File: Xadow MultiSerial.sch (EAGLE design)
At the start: 45 parts, among them J1 12p 0.5mm bottom contact, J2 12p 0.5mm bottom contact, J3 12p 0.5mm bottom contact, J4 12p 0.5mm bottom contact, Q1 MOSFET-N-044020001, Q2 MOSFET-N-044020001, Q3 MOSFET-N-044020001, Q4 MOSFET-N-044020001, Q5 MOSFET-N-044020001, Q6 MOSFET-N-044020001, U1 SC16IS752, X1 CTS_32X25_SMD

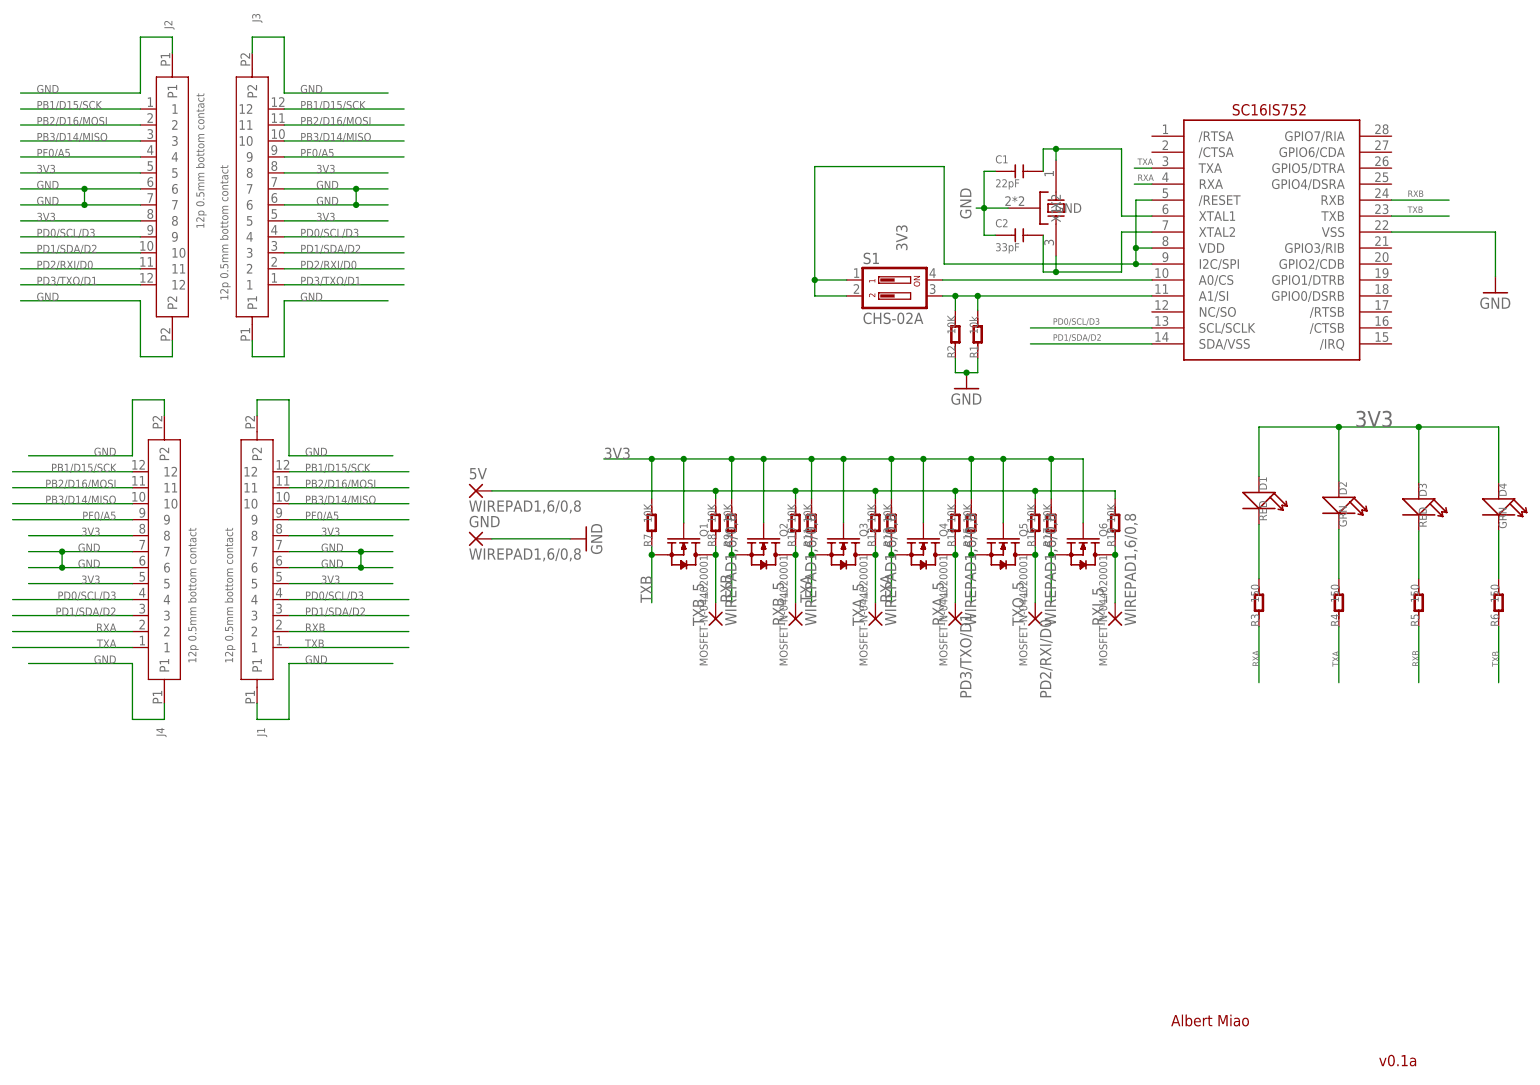
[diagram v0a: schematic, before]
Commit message: Fixed errors and relayed out, last attempt with MOSFET level shifter, need to try TXS shifter
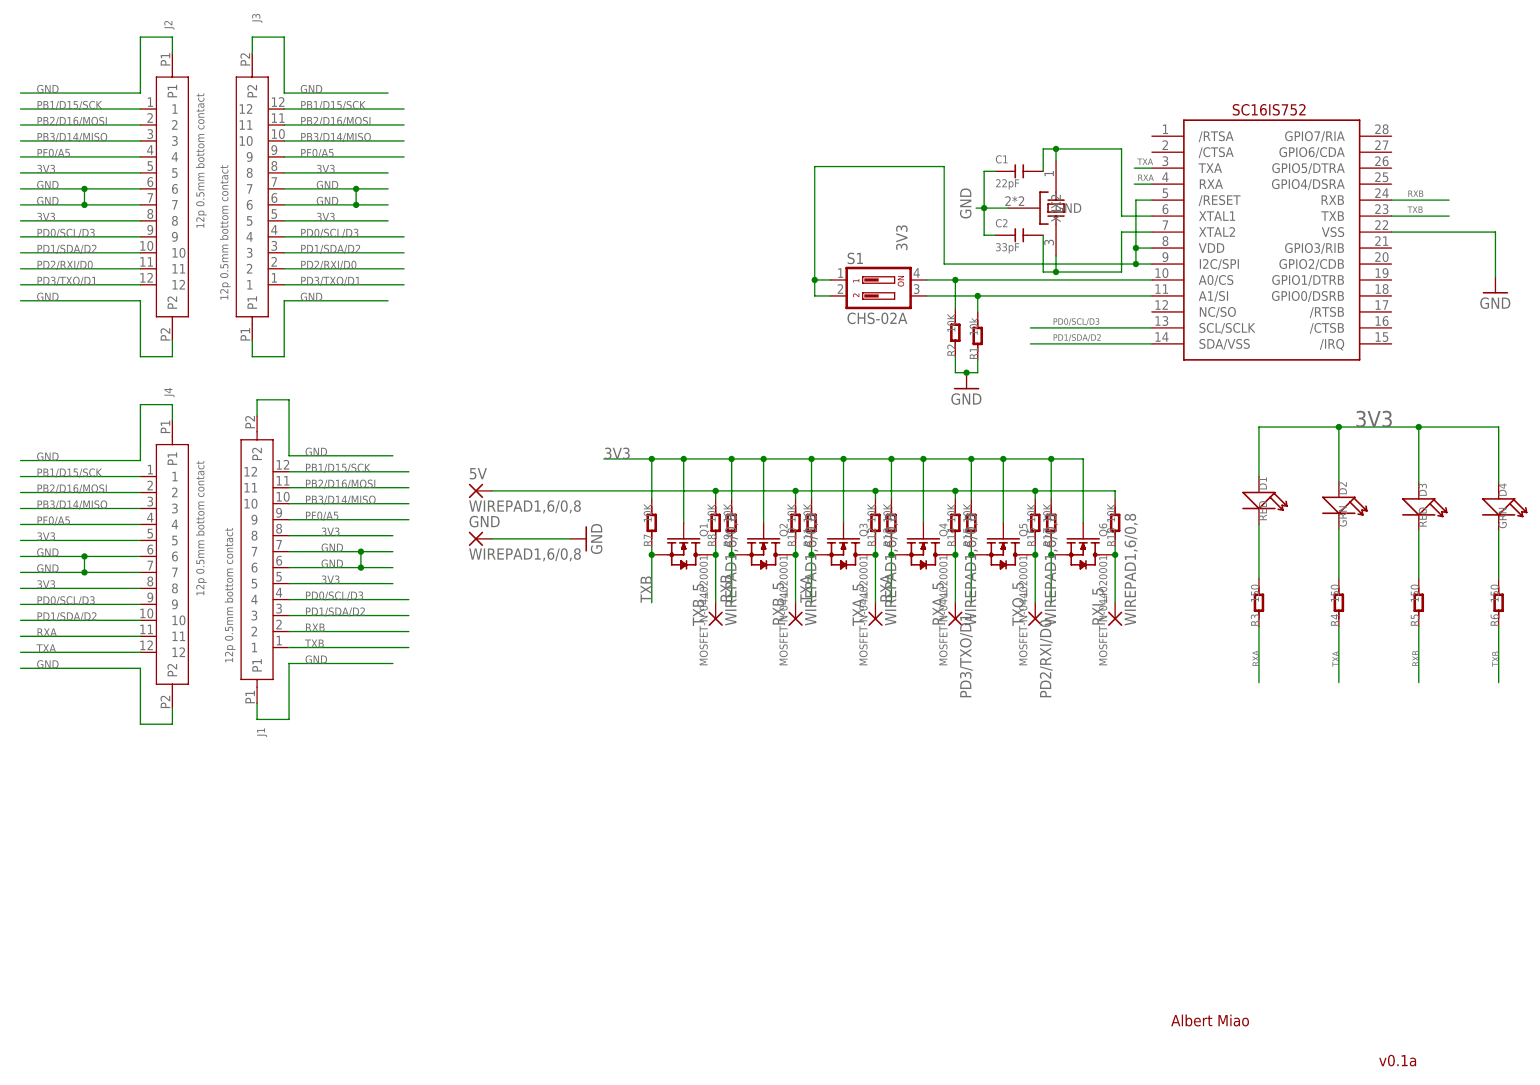
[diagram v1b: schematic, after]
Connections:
- net N$3: no longer R2.2
- net N$5: now also R2.2
- net PB1/D15/SCK: now also J4.1; no longer J4.12
- net PB2/D16/MOSI: now also J4.2; no longer J4.11
- net PB3/D14/MISO: now also J4.3; no longer J4.10
- net PD0/SCL/D3: now also J4.9; no longer J4.4
- net PD1/SDA/D2: now also J4.10; no longer J4.3
- net PF0/A5: now also J4.4; no longer J4.9
- net RXA: now also J4.11; no longer J4.2
- net TXA: now also J4.12; no longer J4.1
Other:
- moved on the sheet: J4, S1

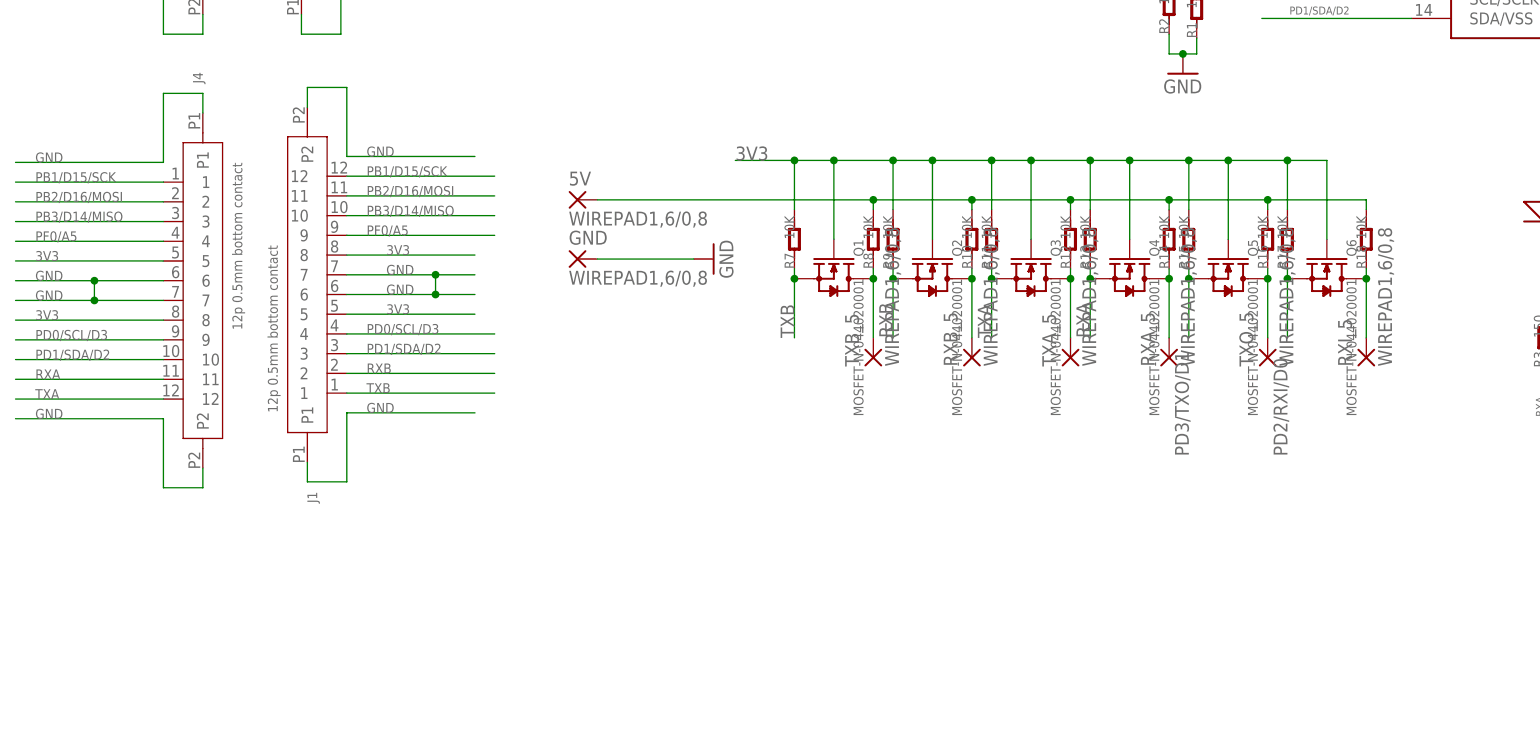
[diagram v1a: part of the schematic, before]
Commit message: Added TXS based level translation
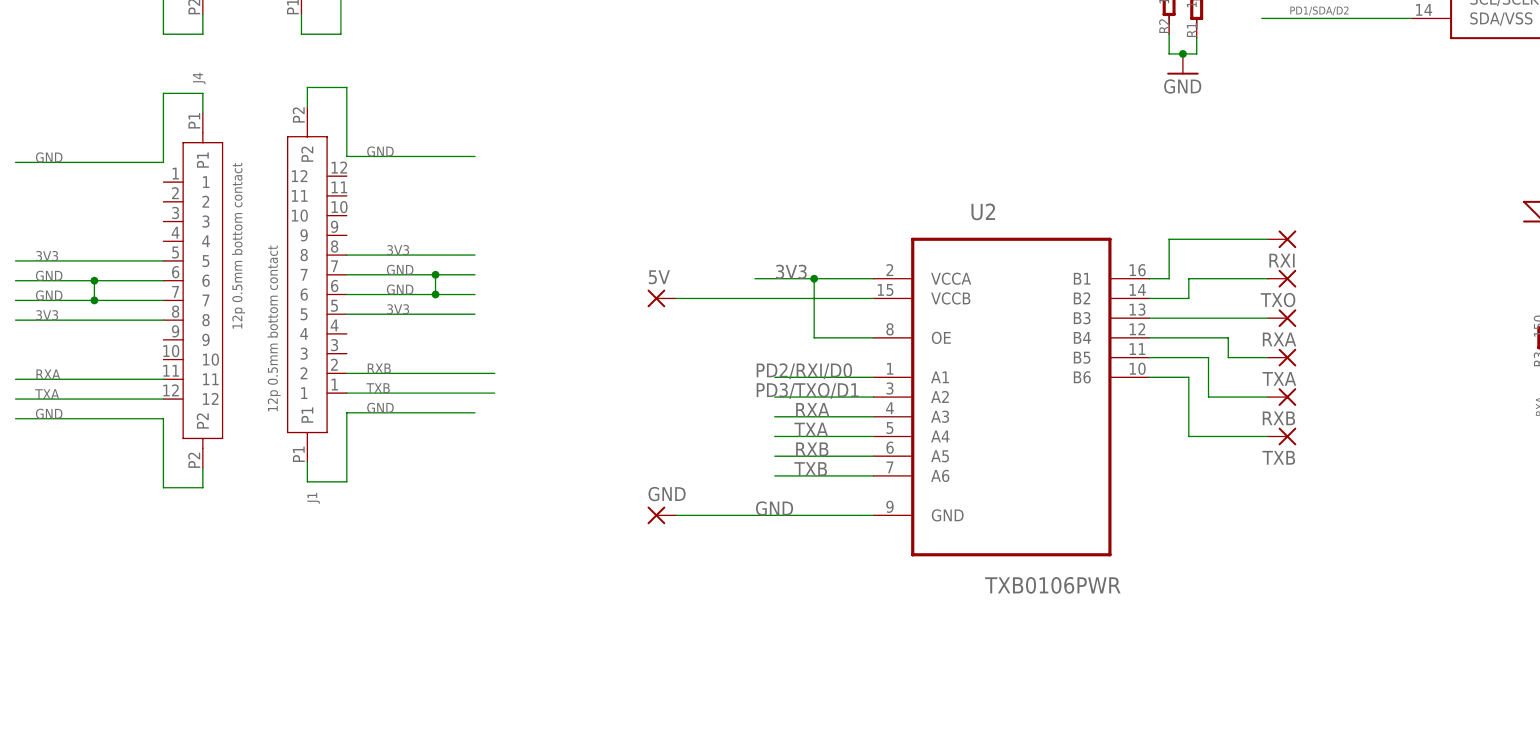
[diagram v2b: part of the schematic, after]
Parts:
- removed Q1, Q2, Q3, Q4, Q5, Q6: MOSFET-N-044020001, OPL:MOSFET-N-044020001
- removed R10, R11, R12, R13, R14, R15, R16, R17, R18, R7, R8, R9: 10K, OPL:R-0603
- removed RXA_5, RXB_5, RXI_5, TXA_5, TXB_5, TXO_5: WIREPAD1,6/0,8, wirepad:WIREPAD1,6/0,8
- added RXA, RXB, RXI, TXA, TXB, TXO: (no value), wirepad:1,6/0,8
- added U2: TXB0106PWR, Texas Instruments_By_element14_Batch_1:TXB0106PWR
- 5V, GND: value WIREPAD1,6/0,8 -> (none); device wirepad:WIREPAD1,6/0,8 -> wirepad:1,6/0,8
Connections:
- removed net N$17: 5V.P, R10.2, R12.2, R14.2, R16.2, R18.2, R8.2
- new net N$4: 5V.P, U2.VCCB
- net 3V3: now also U2.OE, U2.VCCA; no longer Q1.G, Q2.G, Q3.G, Q4.G, Q5.G, Q6.G, R11.2, R13.2, R15.2, R17.2, R7.2, R9.2
- net GND: now also U2.GND
- net N$18: now also RXI.P, U2.B1; no longer Q1.D, R8.1, TXB_5.P
- net N$19: now also TXO.P, U2.B2; no longer Q2.D, R10.1, RXB_5.P
- net N$20: now also RXA.P, U2.B3; no longer Q3.D, R12.1, TXA_5.P
- net N$21: now also TXA.P, U2.B4; no longer Q4.D, R14.1, RXA_5.P
- net N$22: now also RXB.P, U2.B5; no longer Q5.D, R16.1, TXO_5.P
- net N$23: now also TXB.P, U2.B6; no longer Q6.D, R18.1, RXI_5.P
- net PB1/D15/SCK: no longer J1.12, J4.1
- net PB2/D16/MOSI: no longer J1.11, J4.2
- net PB3/D14/MISO: no longer J1.10, J4.3
- net PD0/SCL/D3: no longer J1.4, J4.9
- net PD1/SDA/D2: no longer J1.3, J4.10
- net PD2/RXI/D0: now also U2.A1; no longer Q6.S, R17.1
- net PD3/TXO/D1: now also U2.A2; no longer Q5.S, R15.1
- net PF0/A5: no longer J1.9, J4.4
- net RXA: now also U2.A3; no longer Q4.S, R13.1
- net RXB: now also U2.A5; no longer Q2.S, R9.1
- net TXA: now also U2.A4; no longer Q3.S, R11.1
- net TXB: now also U2.A6; no longer Q1.S, R7.1
